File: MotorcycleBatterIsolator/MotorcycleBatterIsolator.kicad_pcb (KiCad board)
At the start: 0 parts

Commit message: Finally onto the PCB. SHould just be a route job then sending it off
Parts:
- added BZ1: Buzzer, Buzzer_Beeper:MagneticBuzzer_ProSignal_ABT-410-RC, F.Cu at (107.8, 136.2)
- added C1: 1uf, Capacitor_SMD:C_0603_1608Metric, F.Cu at (132.4, 165.3)
- added C10: 4.7pF, Capacitor_SMD:C_0603_1608Metric, F.Cu at (151.2, 126.1)
- added C11: 100nf, Capacitor_SMD:C_0603_1608Metric, F.Cu at (147.8, 122.1)
- added C12: 1uf, Capacitor_SMD:C_0603_1608Metric, F.Cu at (134.5, 120.6)
- added C13: 100nf, Capacitor_SMD:C_0603_1608Metric, F.Cu at (143.0, 119.6)
- added C14: 100nf, Capacitor_SMD:C_0603_1608Metric, F.Cu at (137.8, 119.6)
- added C15: 1uf, Capacitor_SMD:C_0603_1608Metric, F.Cu at (134.5, 118.8)
- added C16: 10uf, Capacitor_SMD:C_0603_1608Metric, F.Cu at (125.7, 135.2)
- added C17: 100nf, Capacitor_SMD:C_0603_1608Metric, F.Cu at (134.5, 125.8)
- added C18: 100nf, Capacitor_SMD:C_0603_1608Metric, F.Cu at (147.8, 123.8)
- added C19: 10uf, Capacitor_SMD:C_0603_1608Metric, F.Cu at (128.8, 135.2)
- added C2: 22uF, Capacitor_SMD:C_0805_2012Metric, F.Cu at (143.4, 166.8)
- added C20: 100nf, Capacitor_SMD:C_0603_1608Metric, F.Cu at (142.0, 131.3)
- added C21: 100nf, Capacitor_SMD:C_0603_1608Metric, F.Cu at (139.8, 131.3)
- added C22: 100nf, Capacitor_SMD:C_0603_1608Metric, F.Cu at (138.0, 131.3)
- added C3: 10uf, Capacitor_SMD:C_0603_1608Metric, F.Cu at (131.8, 135.2)
- added C4: 10uf, Capacitor_SMD:C_0603_1608Metric, F.Cu at (134.8, 135.2)
- added C5: 1uf, Capacitor_SMD:C_0603_1608Metric, F.Cu at (135.2, 115.8)
- added C6: 100nf, Capacitor_SMD:C_0603_1608Metric, F.Cu at (125.0, 119.6)
- added C7: 4.7pF, Capacitor_SMD:C_0603_1608Metric, F.Cu at (151.2, 129.3)
- added C8: 1uf, Capacitor_SMD:C_0603_1608Metric, F.Cu at (148.2, 138.0)
- added C9: 100nf, Capacitor_SMD:C_0603_1608Metric, F.Cu at (134.5, 127.6)
- added D1: D, Diode_SMD:D_SMA, F.Cu at (120.5, 139.2)
- added D10: D, Diode_SMD:D_SMA, F.Cu at (121.0, 131.8)
- added D11: LED, LED_SMD:LED_0603_1608Metric, F.Cu at (132.0, 115.8)
- added D12: D_Zener, Diode_SMD:D_MiniMELF, F.Cu at (104.2, 142.2)
- added D13: D_Zener, Diode_SMD:D_MiniMELF, F.Cu at (151.0, 134.5)
- added D2: D, Diode_SMD:D_SMA, F.Cu at (120.5, 135.5)
- added D3: D, Diode_SMD:D_SMA, F.Cu at (120.5, 143.0)
- added D6: LED, LED_SMD:LED_0603_1608Metric, F.Cu at (137.2, 168.8)
- added D7: D, Diode_SMD:D_SMA, F.Cu at (138.8, 139.0)
- added D8: D, Diode_SMD:D_SMA, F.Cu at (139.0, 154.0)
- added D9: LED, LED_SMD:LED_0603_1608Metric, F.Cu at (128.5, 115.8)
- added J1: Conn_01x04, AndersonPowerPole:APP_2x2, F.Cu at (114.1, 153.6)
- added J2: Micro_SD_Card_Det, Connector_Card:microSD_HC_Molex_104031-0811, F.Cu at (143.0, 112.1)
- added J3: Conn_01x06_Female, Connector:Tag-Connect_TC2030-IDC-NL_2x03_P1.27mm_Vertical, F.Cu at (153.0, 120.6)
- added J4: Conn_01x04, AndersonPowerPole:APP_2x2, F.Cu at (135.0, 154.0)
- added J5: USB_C_Receptacle_USB2.0, Connector_USB:USB_C_Receptacle_HRO_TYPE-C-31-M-12, F.Cu at (130.2, 106.5)
- added JP1: Jumper_2_Bridged, Jumper:SolderJumper-2_P1.3mm_Bridged2Bar_Pad1.0x1.5mm, F.Cu at (134.0, 139.8)
- added Q2: Q_NMOS_GDS, Package_TO_SOT_SMD:TO-252-2, F.Cu at (127.5, 164.2)
- added Q3: Q_NMOS_GDS, Package_TO_SOT_SMD:TO-252-2, F.Cu at (120.0, 164.2)
- added Q5: Q_NMOS_GDS, Package_TO_SOT_SMD:TO-252-2, F.Cu at (127.7, 150.8)
- added Q6: Q_NMOS_GDS, Package_TO_SOT_SMD:TO-252-2, F.Cu at (120.2, 150.8)
- added Q7: 2N7002, Package_TO_SOT_SMD:SOT-23, F.Cu at (116.2, 127.5)
- added R1: 2.2M, Resistor_SMD:R_0603_1608Metric, F.Cu at (143.4, 164.5)
- added R10: 10K, Resistor_SMD:R_0603_1608Metric, F.Cu at (119.2, 127.5)
- added R11: 10K, Resistor_SMD:R_0603_1608Metric, F.Cu at (140.5, 168.8)
- added R12: DNP, Resistor_SMD:R_0603_1608Metric, F.Cu at (134.0, 168.8)
- added R13: 1K, Resistor_SMD:R_0603_1608Metric, F.Cu at (125.0, 116.0)
- added R14: 0.001, Resistor_SMD:R_2512_6332Metric, F.Cu at (139.5, 143.0)
- added R15: 10K, Resistor_SMD:R_0603_1608Metric, F.Cu at (154.0, 128.8)
- added R16: DNP, Resistor_SMD:R_0603_1608Metric, F.Cu at (125.0, 125.8)
- added R17: 1K, Resistor_SMD:R_0603_1608Metric, F.Cu at (145.5, 130.8)
- added R18: 27, Resistor_SMD:R_0603_1608Metric, F.Cu at (134.5, 124.1)
- added R19: 27, Resistor_SMD:R_0603_1608Metric, F.Cu at (134.5, 122.3)
- added R20: 5k1, Resistor_SMD:R_0603_1608Metric, F.Cu at (127.4, 113.1)
- added R21: 5k1, Resistor_SMD:R_0603_1608Metric, F.Cu at (134.2, 112.8)
- added R22: 1K, Resistor_SMD:R_0603_1608Metric, F.Cu at (126.8, 115.8)
- added R23: 5k1, Resistor_SMD:R_0603_1608Metric, F.Cu at (151.5, 138.0)
- added R24: 1K, Resistor_SMD:R_0603_1608Metric, F.Cu at (130.2, 115.8)
- added R25: 5k1, Resistor_SMD:R_0603_1608Metric, F.Cu at (154.5, 142.2)
- added R26: 100K, Resistor_SMD:R_0603_1608Metric, F.Cu at (103.2, 138.5)
- added R27: 10K, Resistor_SMD:R_0603_1608Metric, F.Cu at (103.2, 140.2)
- added R28: 10K, Resistor_SMD:R_0603_1608Metric, F.Cu at (147.8, 120.2)
- added R29: 100K, Resistor_SMD:R_0603_1608Metric, F.Cu at (148.2, 136.2)
- added R30: 10K, Resistor_SMD:R_0603_1608Metric, F.Cu at (148.2, 134.8)
- added R4: 39, R2030:R2030, F.Cu at (128.2, 140.5)
- added SW1: SW_Push, Button_Switch_SMD:SW_SPST_TL3342, F.Cu at (149.6, 165.8)
- added SW2: SW_Push, Button_Switch_SMD:SW_SPST_TL3342, F.Cu at (119.2, 107.0)
- added SW3: SW_Push, Button_Switch_SMD:SW_SPST_TL3342, F.Cu at (119.2, 120.0)
- added SW4: SW_Push, Button_Switch_SMD:SW_SPST_TL3342, F.Cu at (119.2, 113.5)
- added TH1: Thermistor_NTC, Connector_PinHeader_2.54mm:PinHeader_1x02_P2.54mm_Horizontal, F.Cu at (151.9, 111.5)
- added U1: MIC5014, Package_SO:SOP-8_3.76x4.96mm_P1.27mm, F.Cu at (137.4, 165.1)
- added U2: HT75xx-1-SOT89, Package_TO_SOT_SMD:SOT-89-3, F.Cu at (133.0, 131.2)
- added U3: W25Q128JVS, Package_SO:SOIC-8_5.23x5.23mm_P1.27mm, F.Cu at (129.0, 122.6)
- added U4: INA219AxD, Package_SO:SOIC-8_3.9x4.9mm_P1.27mm, F.Cu at (149.8, 141.8)
- added U5: RP2040, MCU_RaspberryPi_and_Boards:RP2040-QFN-56, F.Cu at (140.8, 125.0)
- added U6: HT75xx-1-SOT89, Package_TO_SOT_SMD:SOT-89-3, F.Cu at (127.5, 131.2)
- added Y1: 12M, Crystal:Crystal_SMD_5032-2Pin_5.0x3.2mm, F.Cu at (148.5, 128.1)
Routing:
- net /Motorcycle+: track 0.00 -> 72.8 mm
- net Net-(D6-A): track 0.00 -> 59.0 mm
- net Net-(Q2-S): track 0.00 -> 51.8 mm, vias 0 -> 3
- net Net-(U4-IN-): track 0.00 -> 30.1 mm
- net GND: track 0.00 -> 23.9 mm, vias 0 -> 2
- net +12V: track 0.00 -> 23.1 mm
- net /USB_D+: track 0.00 -> 20.8 mm
- net /USB_D-: track 0.00 -> 19.6 mm
- net /GATE_CTRL: track 0.00 -> 16.9 mm
- net /Battery+: track 0.00 -> 15.2 mm
- net Net-(D3-K): track 0.00 -> 4.77 mm
- net Net-(JP1-A): track 0.00 -> 3.81 mm
- net Net-(D6-K): track 0.00 -> 1.64 mm
- net Net-(U5-USB_DM): track 0.00 -> 1.22 mm
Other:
- board outline added: 77.5 x 67.5 mm
- copper layers 0 -> 2

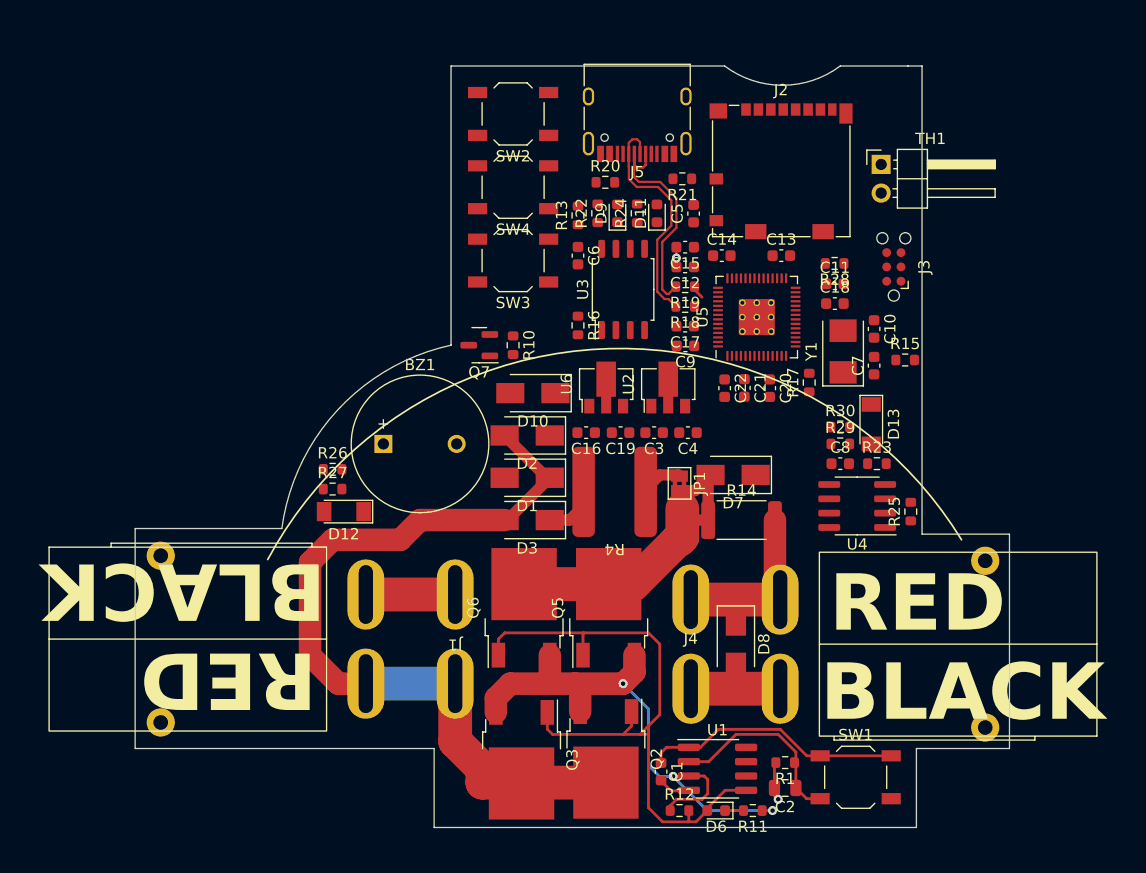
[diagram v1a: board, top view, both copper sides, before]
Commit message: This is the version that got sent off to fab
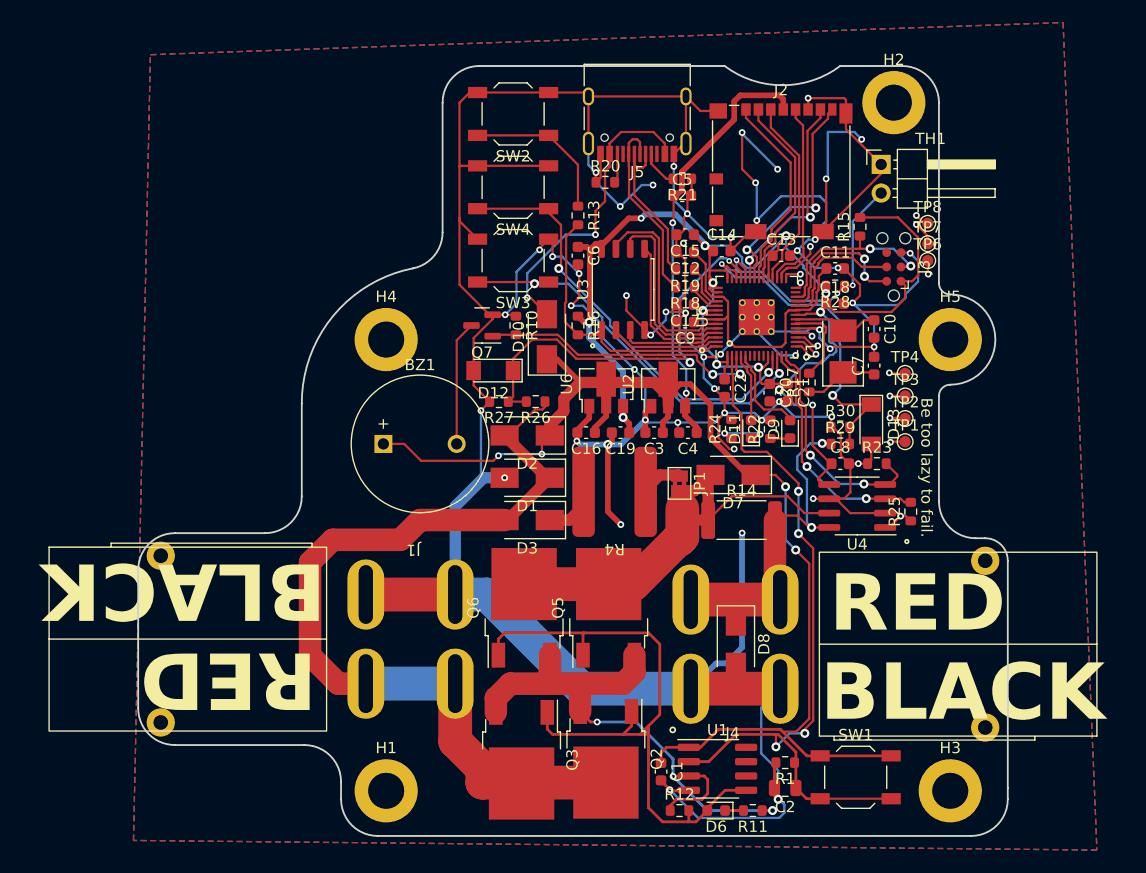
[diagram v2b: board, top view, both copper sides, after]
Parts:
- added G***: LOGO, Logo:Hephestus, B.Cu at (130.3, 147.3)
- added H1: H, MountingHole:MountingHole_3.2mm_M3_DIN965_Pad, F.Cu at (108.0, 167.0)
- added H2: H, MountingHole:MountingHole_3.2mm_M3_DIN965_Pad, F.Cu at (153.0, 106.0)
- added H3: H, MountingHole:MountingHole_3.2mm_M3_DIN965_Pad, F.Cu at (158.0, 167.0)
- added H4: H, MountingHole:MountingHole_3.2mm_M3_DIN965_Pad, F.Cu at (108.0, 127.0)
- added H5: H, MountingHole:MountingHole_3.2mm_M3_DIN965_Pad, F.Cu at (158.0, 127.0)
- added TP1: TestPoint, TestPoint:TestPoint_Pad_D1.0mm, F.Cu at (154.0, 136.1)
- added TP2: TestPoint, TestPoint:TestPoint_Pad_D1.0mm, F.Cu at (154.0, 134.0)
- added TP3: TestPoint, TestPoint:TestPoint_Pad_D1.0mm, F.Cu at (154.0, 132.0)
- added TP4: TestPoint, TestPoint:TestPoint_Pad_D1.0mm, F.Cu at (154.0, 130.0)
- added TP6: TestPoint, TestPoint:TestPoint_Pad_D1.0mm, F.Cu at (156.0, 120.0)
- added TP7: TestPoint, TestPoint:TestPoint_Pad_D1.0mm, F.Cu at (156.0, 118.5)
- added TP8: TestPoint, TestPoint:TestPoint_Pad_D1.0mm, F.Cu at (156.0, 116.7)
- moved D9 24.5 mm to (143.8, 134.9)
- moved R22 24.5 mm to (142.1, 134.9)
- moved D11 20.9 mm to (140.3, 134.9)
- moved R24 20.9 mm to (138.6, 134.9)
- moved R26 19.0 mm to (121.2, 132.5), turned to 180 degrees
- moved D12 18.2 mm to (117.5, 129.8)
- moved R27 16.7 mm to (118.0, 132.5), turned to 180 degrees
- moved R15 12.5 mm to (150.0, 117.0), turned to 90 degrees
- moved D10 5.15 mm to (122.2, 126.8), turned to 90 degrees
- moved C21 3.87 mm to (143.6, 131.7)
- moved C9 2.11 mm to (134.5, 125.5)
- moved R28 2.00 mm to (147.8, 122.2)
- moved C17 1.91 mm to (134.5, 123.9)
- moved C5 1.87 mm to (134.2, 114.2), turned to 0 degrees
- moved Q7 1.77 mm to (116.5, 125.8)
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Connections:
- R27 pad 1: GND -> /MotorcycleVoltage3v3
- R27 pad 2: /MotorcycleVoltage3v3 -> GND
- R28 pad 1: Net-(U5-GPIO28_ADC2) -> /Thermistor
- TH1 pad 2: Net-(U5-GPIO28_ADC2) -> /Thermistor
- U5 pad 13: unconnected-(U5-GPIO10) -> /SDA
- U5 pad 14: unconnected-(U5-GPIO11) -> /SCL
- U5 pad 15: unconnected-(U5-GPIO12) -> Net-(U5-GPIO12)
- U5 pad 16: unconnected-(U5-GPIO13) -> Net-(U5-GPIO13)
- U5 pad 17: unconnected-(U5-GPIO14) -> Net-(U5-GPIO14)
- U5 pad 18: /SD_CLK -> Net-(U5-GPIO15)
- U5 pad 27: /SD_CMD -> Net-(U5-GPIO16)
- U5 pad 28: /DAT3 -> Net-(U5-GPIO17)
- U5 pad 29: /DAT2 -> Net-(U5-GPIO18)
- U5 pad 30: /DAT1 -> Net-(U5-GPIO19)
- U5 pad 31: /DAT0 -> /SD_CLK
- U5 pad 32: unconnected-(U5-GPIO21) -> /SD_CMD
- U5 pad 34: Net-(D11-A) -> /DAT3
- U5 pad 35: Net-(D9-A) -> /DAT2
- U5 pad 36: /SDA -> /DAT1
- U5 pad 37: /SCL -> /DAT0
- U5 pad 38: /MotorcycleVoltage3v3 -> /Thermistor
- U5 pad 39: /BatteryVoltage3v3 -> /MotorcycleVoltage3v3
- U5 pad 4: unconnected-(U5-GPIO2) -> Net-(D11-A)
- U5 pad 40: Net-(U5-GPIO28_ADC2) -> /BatteryVoltage3v3
- U5 pad 5: unconnected-(U5-GPIO3) -> Net-(D9-A)
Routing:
- net GND: track 23.9 -> 460.5 mm, vias 2 -> 54
- net +3V3: track 0.00 -> 139.7 mm, vias 0 -> 13
- net +12V: track 23.1 -> 107.2 mm, vias 0 -> 4
- net /GATE_CTRL: track 16.9 -> 65.3 mm, vias 0 -> 4
- net Net-(U5-GPIO8): track 0.00 -> 38.5 mm, vias 0 -> 2
- net Net-(J2-VDD): track 0.00 -> 38.3 mm, vias 0 -> 2
- net /MotorcycleVoltage3v3: track 0.00 -> 36.9 mm, vias 0 -> 2
- net Net-(U5-GPIO9): track 0.00 -> 35.6 mm, vias 0 -> 2
- net /BatteryVoltage3v3: track 0.00 -> 29.6 mm, vias 0 -> 2
- net +1V1: track 0.00 -> 27.5 mm
- net Net-(D10-A): track 0.00 -> 27.3 mm, vias 0 -> 2
- net /BUZZER_CTRL: track 0.00 -> 25.4 mm, vias 0 -> 2
- net Net-(U3-~{CS}): track 0.00 -> 24.9 mm
- net /Thermistor: track 0.00 -> 24.1 mm, vias 0 -> 3
- net /SDA: track 0.00 -> 21.4 mm, vias 0 -> 2
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- added copper zone on B.Cu, net GND
- added copper zone on F.Cu, net GND
- added copper zone on In1.Cu, net GND
- added copper zone on In2.Cu, net GND
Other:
- board size 77.5 x 67.5 mm -> 77.1 x 68.2 mm
- copper layers 2 -> 4
- board text added: "2022 AB1TJ Battery Disconnector Push lone button to turn on for ~50s"
- board text added: "BAT"
- board text added: "Be too lazy to fail."
- board text added: "MCY"
